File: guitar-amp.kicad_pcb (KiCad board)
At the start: 2 copper layers, 160 x 100 mm, 57 parts, among them J1 Speaker Output, J2 Input, J3 AC Mains, J4 Screw_Terminal_01x02, J5 Screw_Terminal_01x02, J6 Screw_Terminal_01x02, SW1 SW_SPST, T1 Transformer_1P_1S

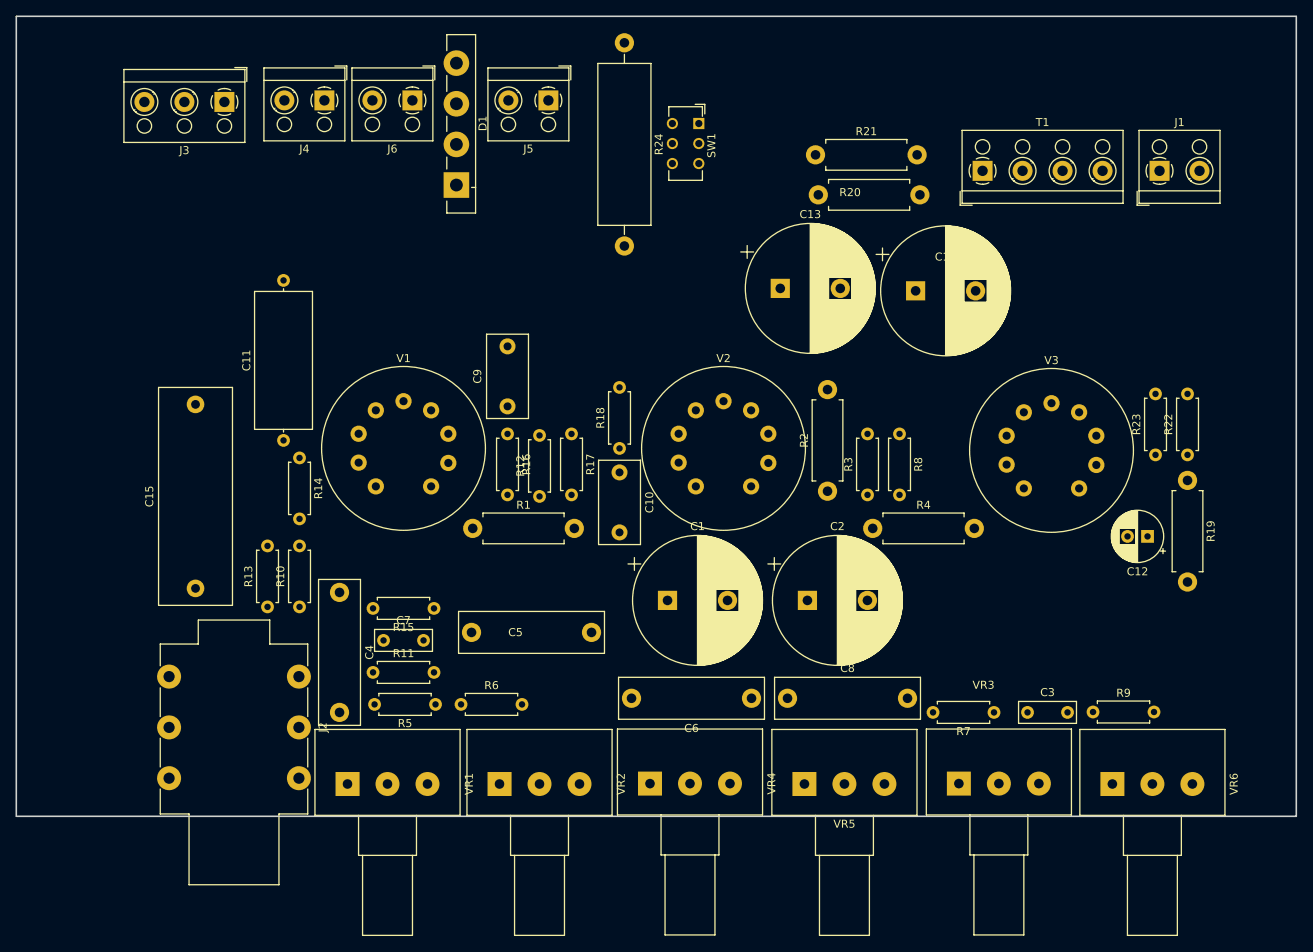
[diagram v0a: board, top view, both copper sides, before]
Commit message: First draft of routing
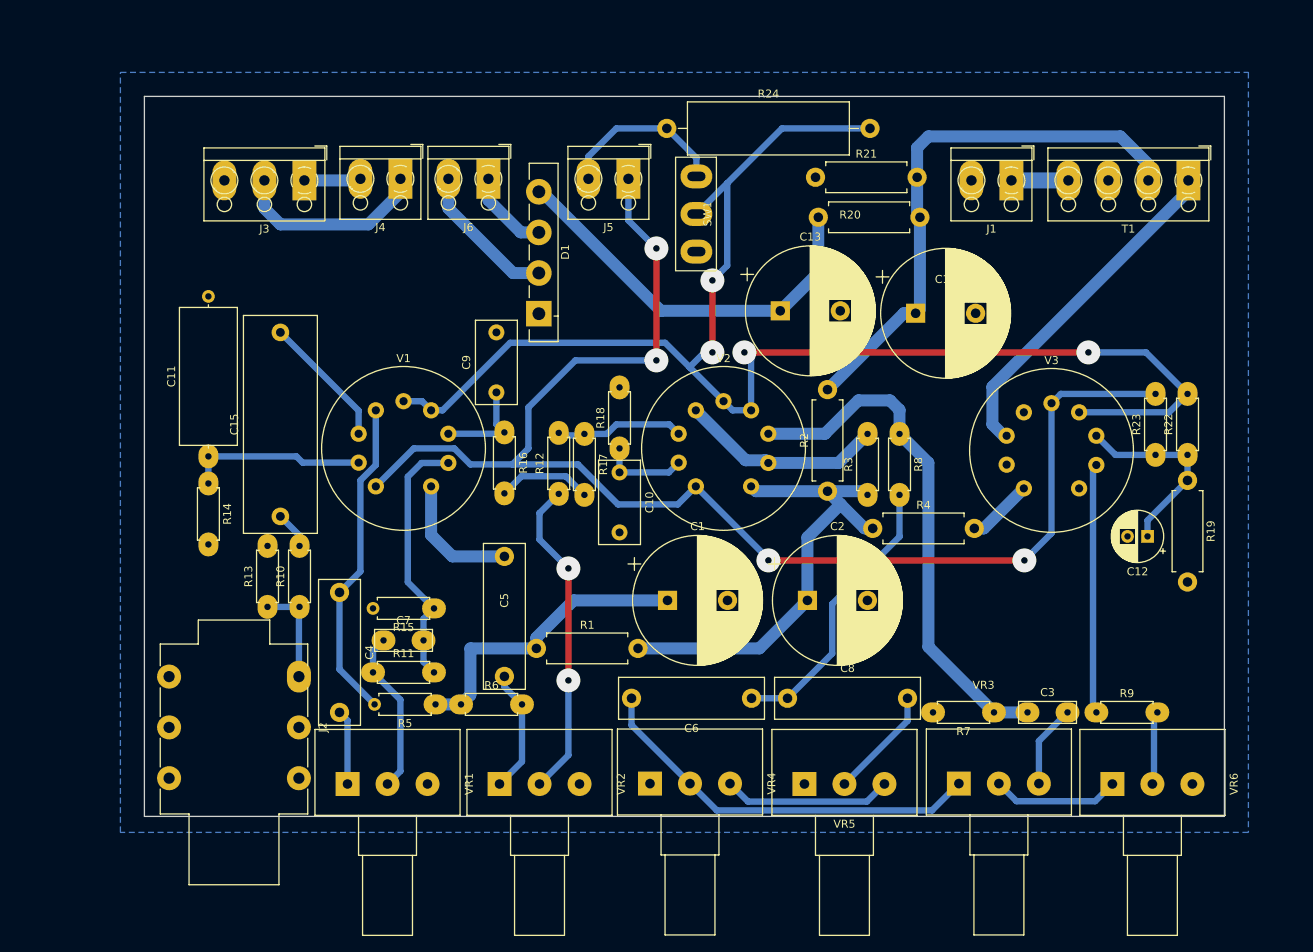
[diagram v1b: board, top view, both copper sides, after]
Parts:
- moved T1 25.8 mm to (246.5, 60.5), turned to 180 degrees
- moved D1 19.1 mm to (165.3, 77.2)
- moved J1 18.5 mm to (224.4, 60.5), turned to 180 degrees
- moved R1 17.0 mm to (165.0, 119.0)
- moved J3 14.0 mm to (136.0, 60.5)
- moved J5 14.0 mm to (176.5, 60.3)
- moved C15 13.9 mm to (133.0, 102.5)
- moved J4 13.7 mm to (148.0, 60.3)
- moved J6 13.7 mm to (159.0, 60.3)
- moved R24 11.9 mm to (181.3, 54.0), turned to 0 degrees
- moved R14 11.8 mm to (124.0, 98.4)
- moved SW1 11.3 mm to (185.0, 64.7)
- moved C5 10.4 mm to (161.0, 107.5), turned to -90 degrees
- moved C11 9.60 mm to (124.0, 95.0)
- moved C13 2.81 mm to (195.5, 76.8)
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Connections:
- net Net-(C1-Pad1) renamed /HighDC_227VDC
- net Net-(C13-Pad1) renamed /HighDC_Prefilter
- net Net-(C14-Pad1) renamed /HighDC_Post
- net Net-(C2-Pad1) renamed /HighDC_241VDC
- net Net-(C3-Pad1) renamed /HighDC_143VDC
- net Net-(C5-Pad1) renamed /HighDC_V1B_Anode
- net Net-(D1-Pad2) renamed /HighDC_Trafo1
- net Net-(D1-Pad3) renamed /HighDC_Trafo2
- net Net-(J3-Pad1) renamed /AC_L
- net Net-(J3-Pad2) renamed /AC_N
- net Net-(R3-Pad2) renamed /HighDC_V2A_Anode
- net Net-(R4-Pad2) renamed /HighDC_GateValve3
- net Net-(T1-Pad1) renamed /HighDC_OT
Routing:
- net Net-(R22-Pad2): track 0.00 -> 182.2 mm, vias 0 -> 4
- net Net-(J5-Pad1): track 0.00 -> 176.1 mm, vias 0 -> 4
- net /HighDC_Post: track 0.00 -> 69.0 mm
- net /HighDC_143VDC: track 0.00 -> 65.5 mm
- net /HighDC_241VDC: track 0.00 -> 60.0 mm
- net Net-(C6-Pad2): track 0.00 -> 50.1 mm
- net /HighDC_Prefilter: track 0.00 -> 50.0 mm
- net /HighDC_OT: track 0.00 -> 43.0 mm
- net Net-(C4-Pad1): track 0.00 -> 40.5 mm
- net Net-(R12-Pad1): track 0.00 -> 40.3 mm, vias 0 -> 2
- net /HighDC_227VDC: track 0.00 -> 38.6 mm
- net Net-(C6-Pad1): track 0.00 -> 35.7 mm
- net Net-(C7-Pad2): track 0.00 -> 32.7 mm
- net Net-(R9-Pad1): track 0.00 -> 31.3 mm
- net /HighDC_V2A_Anode: track 0.00 -> 25.7 mm
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- added copper zone on B.Cu, net Earth
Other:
- board size 160 x 100 mm -> 135 x 90 mm
- board text removed: "TODO: - Softstart switch which footprint? - Softstart resistor which size / footprint?"
